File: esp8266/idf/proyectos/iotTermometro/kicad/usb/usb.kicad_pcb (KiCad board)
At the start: 2 copper layers, 49 x 19.5 mm, 12 parts, among them J1 USB_A, SW1 SW_Push, U1 AMS1117, U2 ESP-12F, U3 S

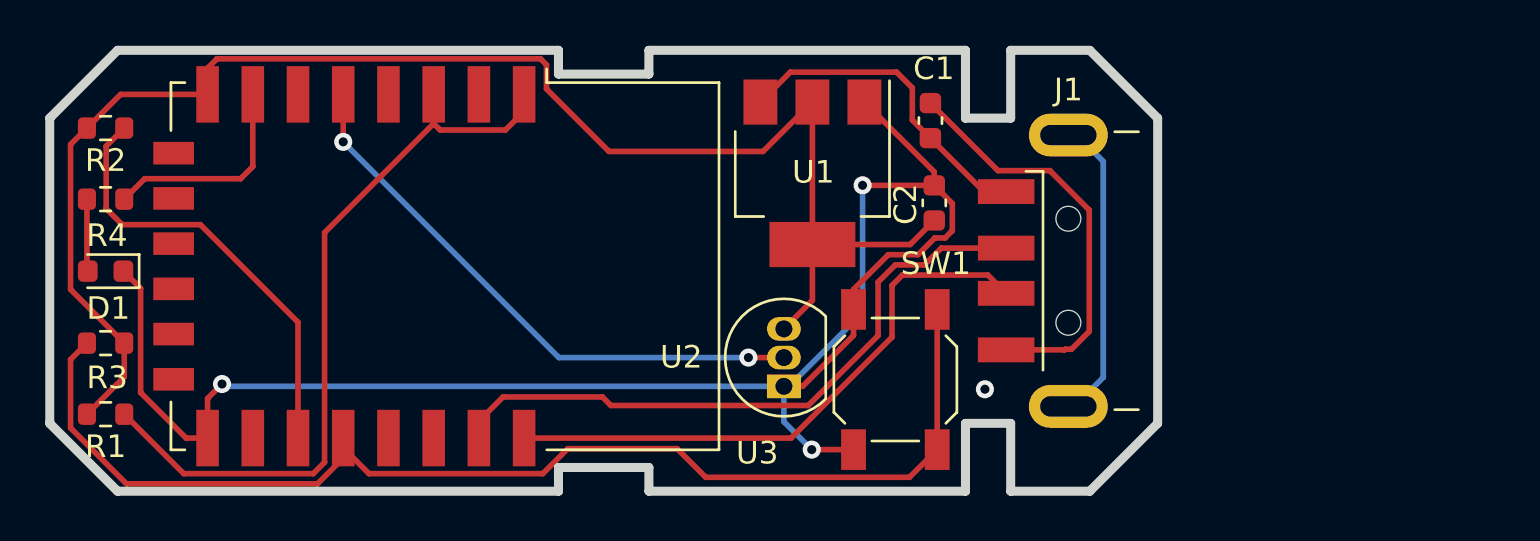
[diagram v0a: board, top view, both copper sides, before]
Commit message: x
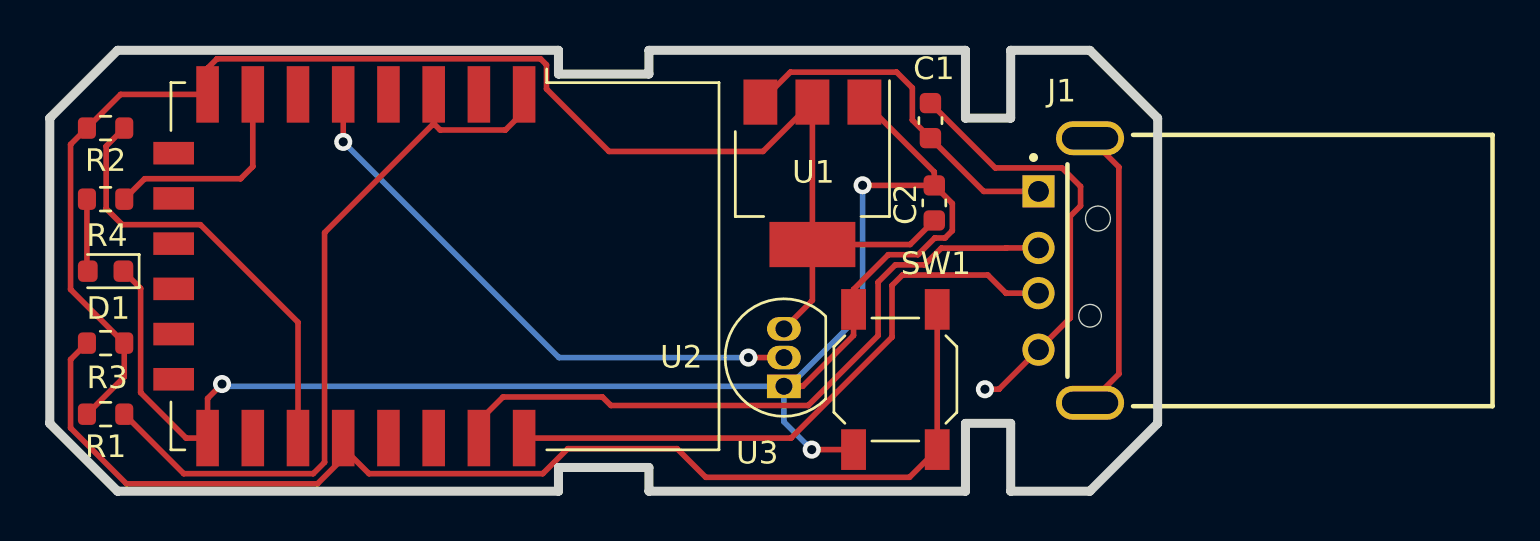
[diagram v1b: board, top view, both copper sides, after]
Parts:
- J1: value USB_A -> USB-AM-S-X-X-TH; footprint Connector_USB:USB_A_CNCTech_1001-011-01101_Horizontal -> conector_usb:SAMTEC_USB-AM-S-X-X-TH
- U1: value AMS1117 -> AMS1117-3.3
- U3: value S -> DS18B20
- moved J1 5.94 mm to (145.0, 79.0), turned to 90 degrees
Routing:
- net unconnected-(J1-PadS1): track 0.00 -> 12.8 mm
- net unconnected-(J1-Pad5): track 12.2 -> 0.00 mm
- net /TX: track 26.0 -> 27.4 mm
- net /RX: track 28.9 -> 30.4 mm
- net /VIN: track 17.2 -> 15.9 mm
- net GND: track 93.0 -> 93.9 mm
